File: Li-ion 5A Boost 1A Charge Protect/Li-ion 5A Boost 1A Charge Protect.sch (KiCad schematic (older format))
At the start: 55 parts, among them J1 USB_C_FEMALE, Q1 BUK6D30-40E, SW1 SW_DPST, U1 AP9101CK6, U2 ECH8695R-TL-W, U3 MCP73833T, U4 PAM2423AECADJR

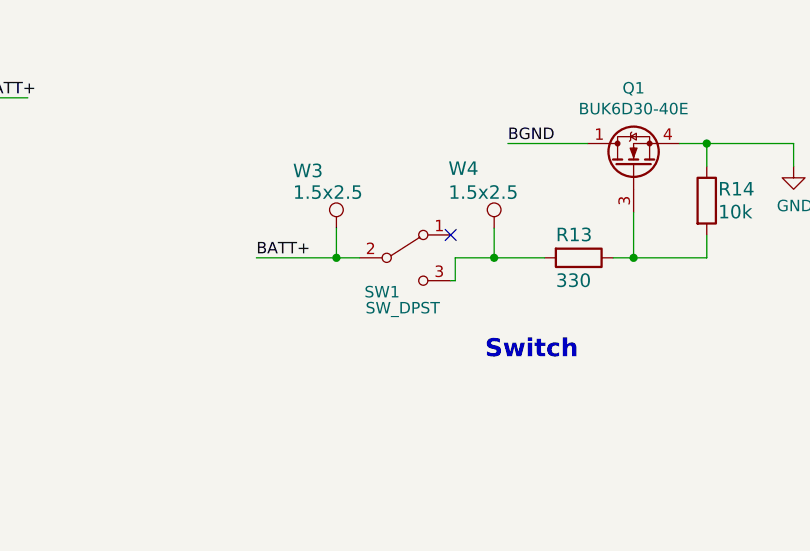
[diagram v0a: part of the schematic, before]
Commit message: Near complete version 1.1.0
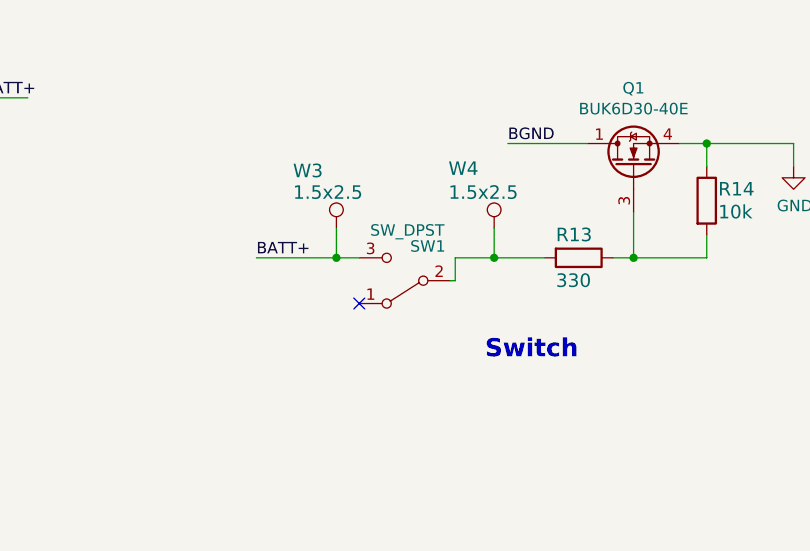
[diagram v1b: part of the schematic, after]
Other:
- moved on the sheet: SW1
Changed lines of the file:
@@
 F 1 "USB_C_FEMALE" H 950 7300 70  0000 L CNN
 F 2 "Connector_LE:GCT_USB4110-GF-A" H 1300 6600 50  0001 C CNN
-F 3 "https://gct.co/files/drawings/usb4125.pdf" H 1300 6600 50  0001 C CNN
+F 3 "https://www.mouser.com/datasheet/2/837/USB4110-1948945.pdf" H 1300 6600 50  0001 C CNN
 F 4 "USB-C Power Female SMD Connector" H 1300 6600 50  0001 C CNN "Description"
 F 5 "2073-USB4110-GF-A-1-ND" H 1300 6600 50  0001 C CNN "Source Part No."
@@
 L Button_Switch_LE:CL-SB-22A SW1
 U 1 1 5EE83AA5
-P 8150 1650
-F 0 "SW1" H 8050 1500 50  0000 C CNN
-F 1 "SW_DPST" H 8140 1430 50  0000 C CNN
-F 2 "Button_Switch_LE:CL-SB-22A_Edge" H 8150 1650 50  0001 C CNN
-F 3 "https://www.nidec-copal-electronics.com/e/catalog/switch/cl-sb.pdf" H 8150 1650 50  0001 C CNN
-F 4 "Slide Switch DPDT Surface Mount, Right Angle" H 8150 1650 50  0001 C CNN "Description"
-F 5 "563-1340-1-ND" H 8150 1650 50  0001 C CNN "Source Part No."
-F 6 "CL-SB-22A-11T" H 8150 1650 50  0001 C CNN "Manufacturer Part No."
-F 7 "Nidec Copal Electronics" H 8150 1650 50  0001 C CNN "Manufacturer Name"
-F 8 "Digikey" H 8150 1650 50  0001 C CNN "Source"
-F 9 "Mouser" H 8150 1650 50  0001 C CNN "Source 2"
-F 10 "229-CL-SB-22A-11T" H 8150 1650 50  0001 C CNN "Source 2 Part No."
-	1    8150 1650
-	1    0    0    -1
+P 8150 1750
+F 0 "SW1" H 8050 1600 50  0000 C CNN
+F 1 "SW_DPST" H 8140 1530 50  0000 C CNN
+F 2 "Button_Switch_LE:CL-SB-22A_Edge" H 8150 1750 50  0001 C CNN
+F 3 "https://www.nidec-copal-electronics.com/e/catalog/switch/cl-sb.pdf" H 8150 1750 50  0001 C CNN
+F 4 "Slide Switch DPDT Surface Mount, Right Angle" H 8150 1750 50  0001 C CNN "Description"
+F 5 "563-1340-1-ND" H 8150 1750 50  0001 C CNN "Source Part No."
+F 6 "CL-SB-22A-11T" H 8150 1750 50  0001 C CNN "Manufacturer Part No."
+F 7 "Nidec Copal Electronics" H 8150 1750 50  0001 C CNN "Manufacturer Name"
+F 8 "Digikey" H 8150 1750 50  0001 C CNN "Source"
+F 9 "Mouser" H 8150 1750 50  0001 C CNN "Source 2"
+F 10 "229-CL-SB-22A-11T" H 8150 1750 50  0001 C CNN "Source 2 Part No."
+	1    8150 1750
+	-1   0    0    1
 $EndComp
 $Comp
@@
 Wire Wire Line
 	9470 1150 9850 1150
-NoConn ~ 8350 1550
+NoConn ~ 7950 1850
 $EndSCHEMATC
